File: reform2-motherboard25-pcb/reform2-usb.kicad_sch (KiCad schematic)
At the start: 74 parts, among them J12 Conn_02x06_Odd_Even, J14 USB_INT2, J17 USB3_A, J5 USB3_A, J6 USB3_A, J9 USB_INT1, U21 SP3012-06UTG, U25 SP3012-06UTG, U26 SP3012-06UTG, U9 TUSB8040PFP, Y1 24MHz

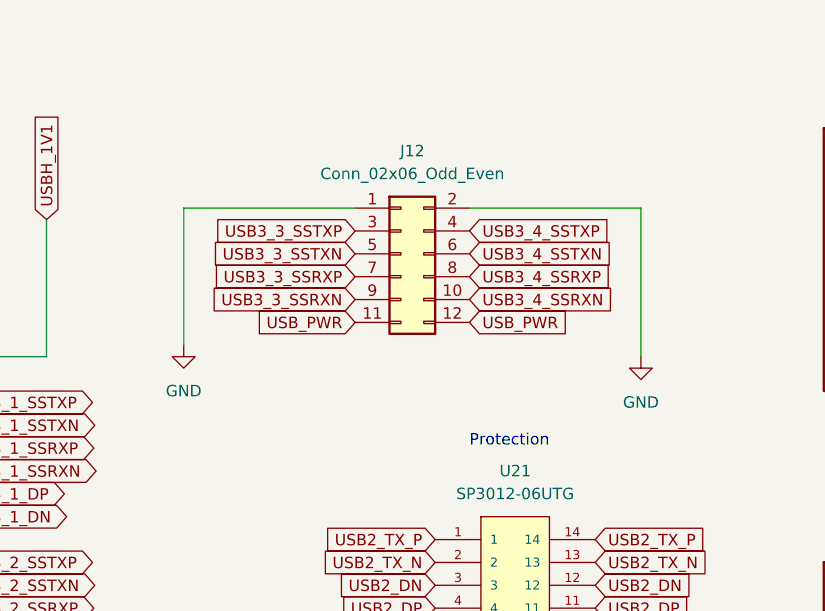
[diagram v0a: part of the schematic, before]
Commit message: motherboard25: r-1 snapshot, ordered for test bringup
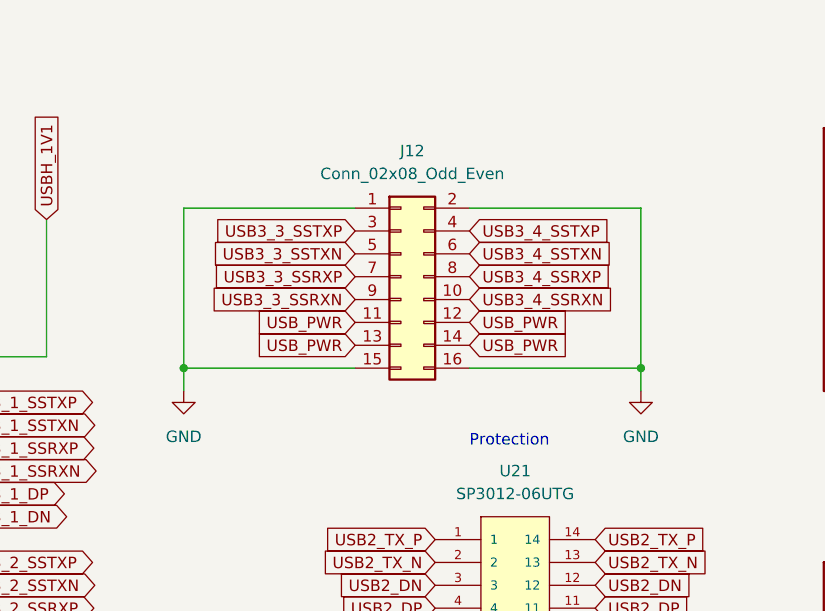
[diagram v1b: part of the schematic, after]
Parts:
- C11, C12, C13, C14, C15, C20, C21, C43, C66, C86, C88, C9, C90: Checked (none) -> y
- C73, C87, C89: Checked (none) -> y; Distributor (none) -> Mouser; LCSC C14445 -> (none); Manufacturer Samsung -> Taiyo Yuden; Manufacturer_No CL05A105KP5NNNC -> UMK107BJ105KA-T
- C91, C92: Checked (none) -> y; Distributor (none) -> Mouser; LCSC C315248 -> (none); Manufacturer Samsung -> Murata; Manufacturer_No CL05A106MP5NUNC -> GRM188R6YA106MA73D
- J12: value Conn_02x06_Odd_Even -> Conn_02x08_Odd_Even; footprint Connector_PinHeader_1.00mm:PinHeader_2x06_P1.00mm_Vertical_SMD -> Connector_PinHeader_1.00mm:PinHeader_2x08_P1.00mm_Vertical_SMD; symbol Connector_Generic:Conn_02x06_Odd_Even -> Connector_Generic:Conn_02x08_Odd_Even; Distributor (none) -> Mouser; Manufacturer (none) -> Harwin; Manufacturer_No (none) -> M40-3200845R
- R59: Checked (none) -> y; Distributor (none) -> Mouser; LCSC C400642 -> (none); Manufacturer Panasonic -> Vishay Dale; Manufacturer_No ERJ2RKF9091X -> CRCW06039K09FKTA
- R60: Checked (none) -> y; Distributor (none) -> Mouser; LCSC C26989 -> (none); Manufacturer UNI-ROYAL -> Vishay Dale; Manufacturer_No 0402WGF9092TCE -> CRCW060390K9FKEA
- R61: Checked (none) -> y; Distributor (none) -> Mouser; LCSC C144787 -> (none); Manufacturer_No AC0402FR-071ML -> RC0603FR-071ML
- R62, R63, R84, R85: Checked (none) -> y; Distributor (none) -> Mouser
- R81: LCSC C242160 -> (none); Manufacturer Panasonic -> Vishay Dale; Manufacturer_No ERJ2GE0R00X -> CRCW06030000Z0EAC
- U21, U25, U26: Field12 0.5 -> (none); Field13 0.0 -> (none); Field14 3.4 -> (none); Field15 02/23/17 -> (none); Field17 0.55 -> (none); Field18 0.25 -> (none); Field21 0.35 -> (none); Field22 0.55mm -> (none); Field23 0.2 -> (none); Field25 14.0 -> (none); Field28 0.15 -> (none); Field30 0.25 -> (none); Field33 3.6 -> (none); Field34 0.0 -> (none); Field38 IPC 7351B -> (none); Field39 1.35 -> (none); Field40 3.5 -> (none); Field42 Littelfuse -> (none); Field43 0.3 -> (none); Field5 1.45 -> (none); Field6 1.25 -> (none)
- U9: Checked (none) -> y; Distributor (none) -> TI
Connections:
- net GND: now also J12.15 (Pin_15), J12.16 (Pin_16)
- net USB_PWR: now also J12.13 (Pin_13), J12.14 (Pin_14)
